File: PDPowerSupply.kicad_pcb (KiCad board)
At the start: 4 copper layers, 35 x 65 mm, 33 parts, among them J1 USB_C_Receptacle_USB2.0_16P, J2 Barrel_Jack_Switch, J3 Barrel_Jack_Switch, J4 Barrel_Jack_Switch, J5 Barrel_Jack_Switch, J6 Barrel_Jack_Switch, J7 Barrel_Jack_Switch, J8 Barrel_Jack_Switch, Q2 Q_PMOS_GDS, U1 CH224K

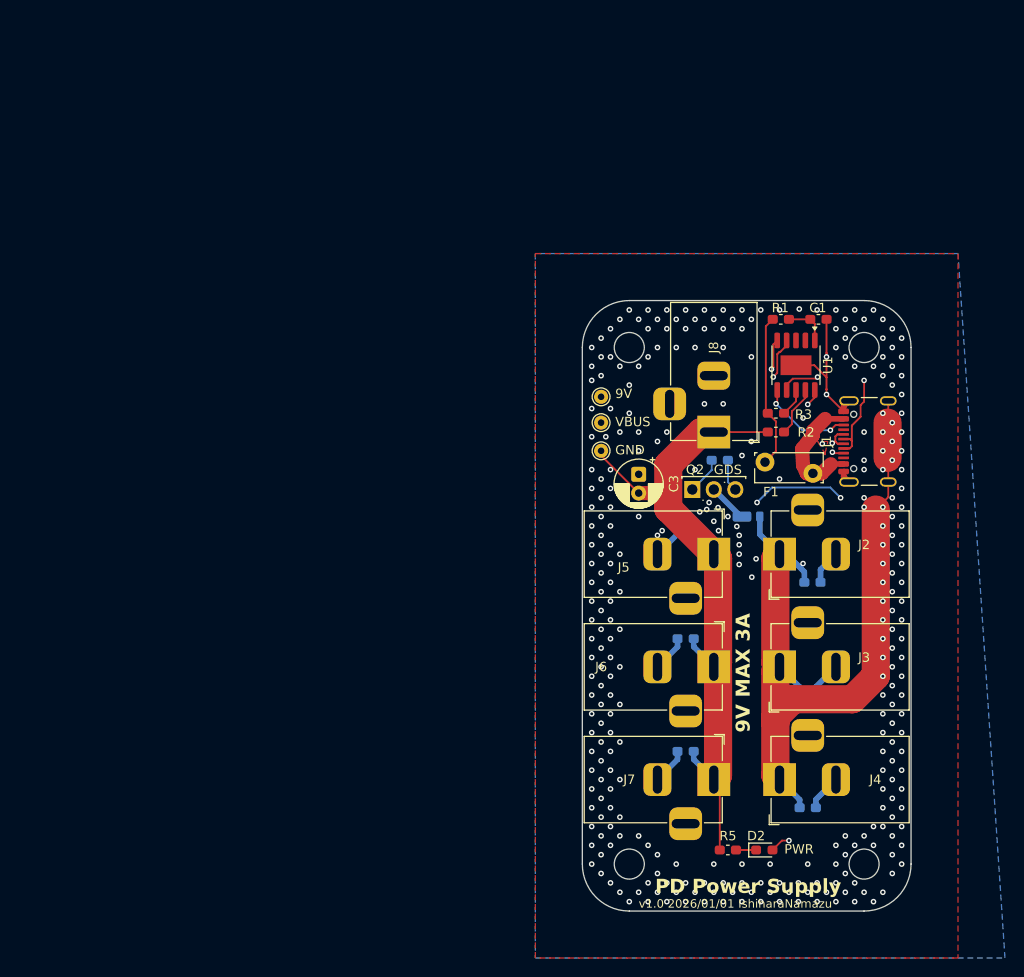
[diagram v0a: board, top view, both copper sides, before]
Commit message: v2.0発注
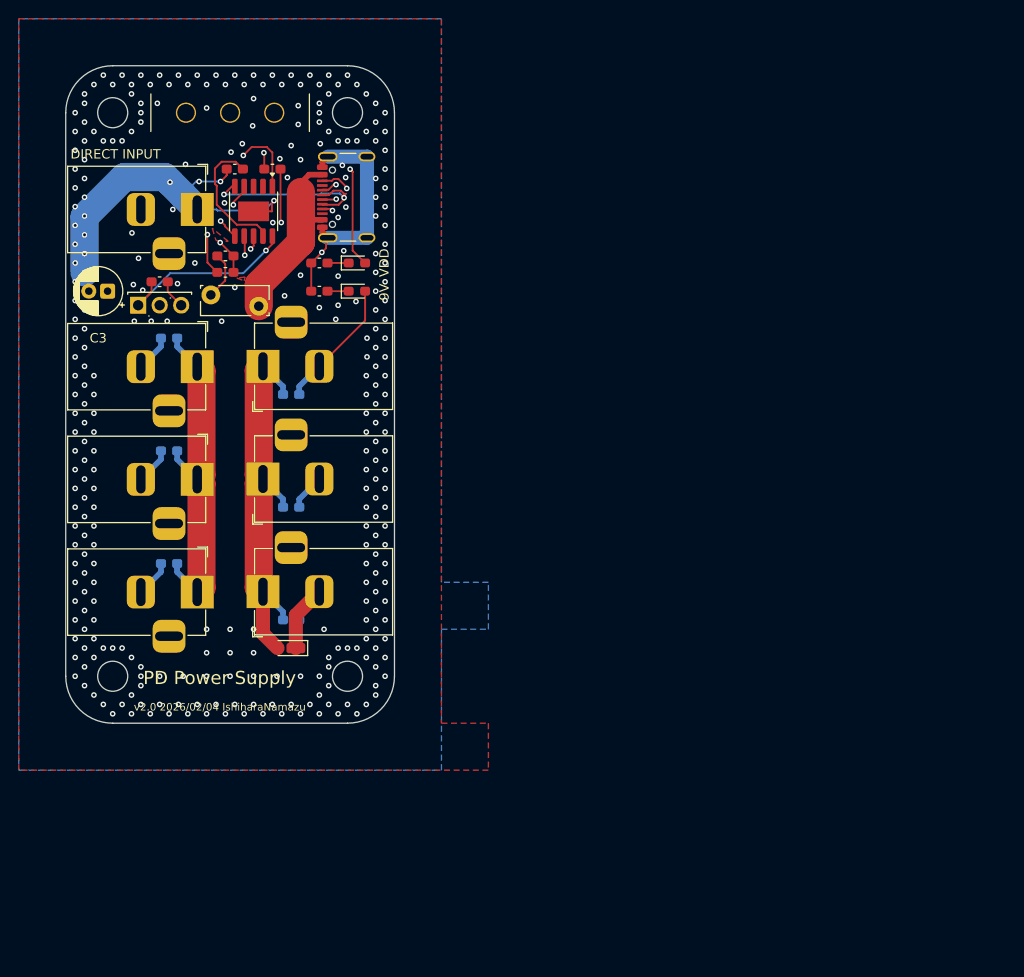
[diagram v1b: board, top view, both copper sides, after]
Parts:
- removed MH1, MH2, MH3, MH4: MountingHole_3.2mm_M3, MountingHole:MountingHole_3.2mm_M3
- removed TP1, TP2, TP4: TestPoint, TestPoint:TestPoint_THTPad_D1.5mm_Drill0.7mm
- added D3: VDD_LED, LED_SMD:LED_0603_1608Metric_Pad1.05x0.95mm_HandSolder, F.Cu at (131.0, 71.0)
- added R6: 470R, Capacitor_SMD:C_0603_1608Metric_Pad1.08x0.95mm_HandSolder, F.Cu at (127.0, 71.0)
- added REF1: MountingHole_3.2mm_M3, MountingHole:MountingHole_3.2mm_M3, F.Cu at (105.0, 55.0)
- added REF2: MountingHole_3.2mm_M3, MountingHole:MountingHole_3.2mm_M3, F.Cu at (130.0, 55.0)
- added REF3: MountingHole_3.2mm_M3, MountingHole:MountingHole_3.2mm_M3, F.Cu at (130.0, 115.0)
- added REF4: MountingHole_3.2mm_M3, MountingHole:MountingHole_3.2mm_M3, F.Cu at (105.0, 115.0)
- added SW1: SW_SPDT, Ishihalib:ROCKERSW_3MS1J102M2QES, F.Cu at (117.5, 55.0)
- D1, R4: moved to F.Cu
- moved R5 73.7 mm to (127.0, 74.0)
- moved D2 73.6 mm to (131.0, 74.0)
- moved C6 70.4 mm to (124.0, 85.0)
- moved C4 69.9 mm to (111.0, 91.0), turned to 180 degrees
- moved C5 69.4 mm to (111.0, 103.0), turned to 180 degrees
- moved J2 65.1 mm to (114.0, 82.0), turned to 0 degrees
- moved J3 65.1 mm to (114.0, 94.0), turned to 0 degrees
- moved J4 65.1 mm to (114.0, 106.0), turned to 0 degrees
- moved R2 64.1 mm to (118.0, 61.0)
- moved C1 63.3 mm to (117.0, 72.0), turned to 180 degrees
- moved R4 62.6 mm to (110.0, 73.0)
- moved Q2 62.2 mm to (107.7, 75.5)
- moved F1 61.6 mm to (120.5, 75.6)
- moved J1 61.3 mm to (131.0, 64.0)
- moved U1 60.0 mm to (120.0, 65.5)
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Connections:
- C3 pad 1: Net-(Q2-S) -> +9V
- F1 pad 1: VBUS -> Net-(F1-Pad1)
- J1 pad A4: VBUS -> Net-(F1-Pad1)
- J1 pad A9: VBUS -> Net-(F1-Pad1)
- J1 pad B4: VBUS -> Net-(F1-Pad1)
- J1 pad B9: VBUS -> Net-(F1-Pad1)
- J8 pad 2: VBUS -> VDD
- J8 pad 3: unconnected-(J8-Pad3) -> /JACK_B
- Q2 pad 2: +9V -> /JACK_B
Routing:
- net VDD: track 0.00 -> 44.9 mm, vias 0 -> 1
- net VBUS: track 43.1 -> 0.00 mm
- net +9V: track 170.6 -> 146.9 mm, vias 14 -> 0
- net Net-(F1-Pad1): track 0.00 -> 20.2 mm
- net Net-(U1-VDD): track 4.72 -> 21.4 mm, vias 0 -> 2
- net GND: track 225.5 -> 211.9 mm, vias 303 -> 313
- net /JACK_B: track 0.00 -> 11.8 mm
- net Net-(U1-VBUS): track 3.00 -> 14.1 mm, vias 0 -> 2
- net Net-(J1-CC2): track 10.1 -> 20.3 mm
- net Net-(U1-CFG1): track 5.42 -> 14.2 mm
- net Net-(Q2-S): track 36.9 -> 28.5 mm, vias 0 -> 1
- net Net-(U1-DM): track 23.7 -> 20.6 mm
- net Net-(D3-K): track 0.00 -> 2.26 mm
- net /PG: track 21.9 -> 20.9 mm
- net Net-(J1-CC1): track 14.6 -> 15.3 mm
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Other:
- board size 35 x 65 mm -> 35 x 70 mm
- board text added: "DIRECT INPUT"
- board text added: "VDD"
- board text added: "v2.0 2026/02/04 IshiharaNamazu"
- board text removed: "9V MAX 3A"
- board text removed: "GDS"
- board text removed: "GND"
- board text removed: "PWR"
- board text removed: "VBUS"
- board text removed: "v1.0 2026/01/01 IshiharaNamazu"
